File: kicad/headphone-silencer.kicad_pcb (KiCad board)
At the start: 2 copper layers, 61 x 12 mm, 6 parts, among them J1 AudioJack3, J2 AudioJack3

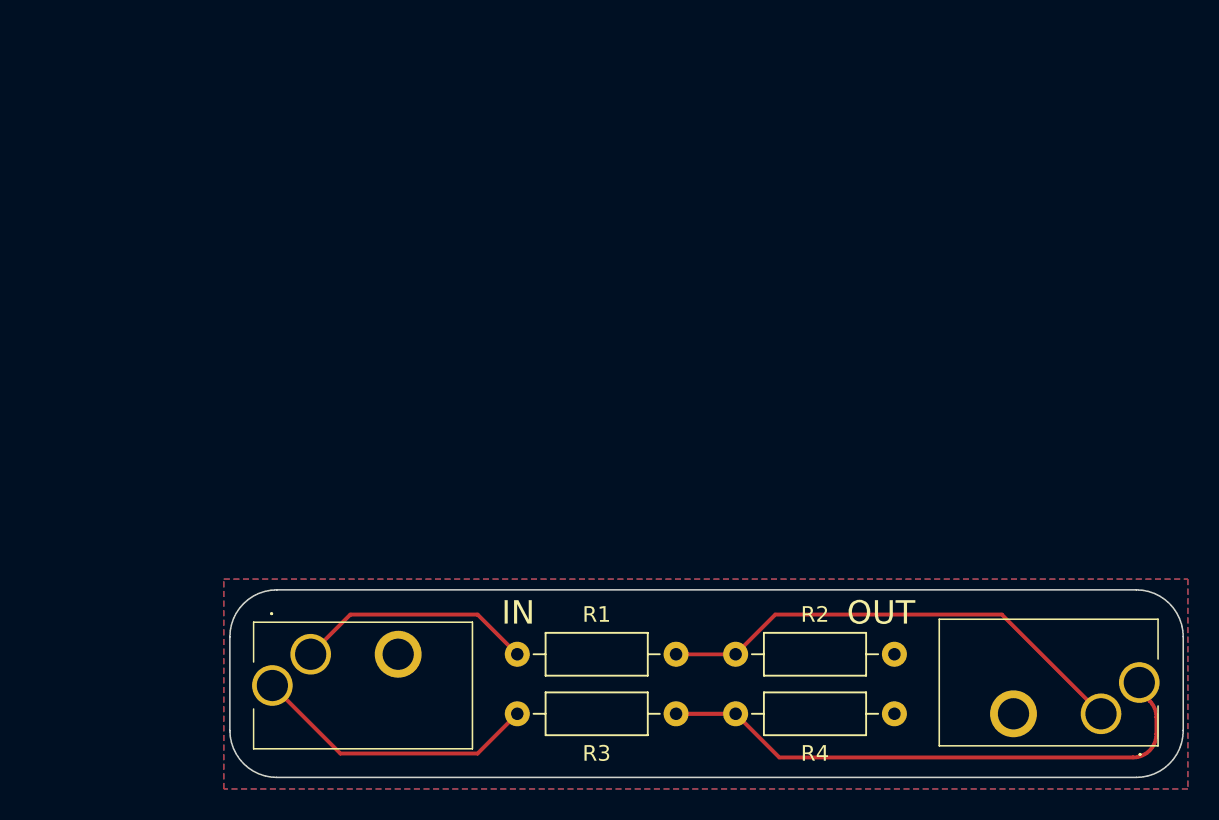
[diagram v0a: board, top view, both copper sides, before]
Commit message: Add pdfs
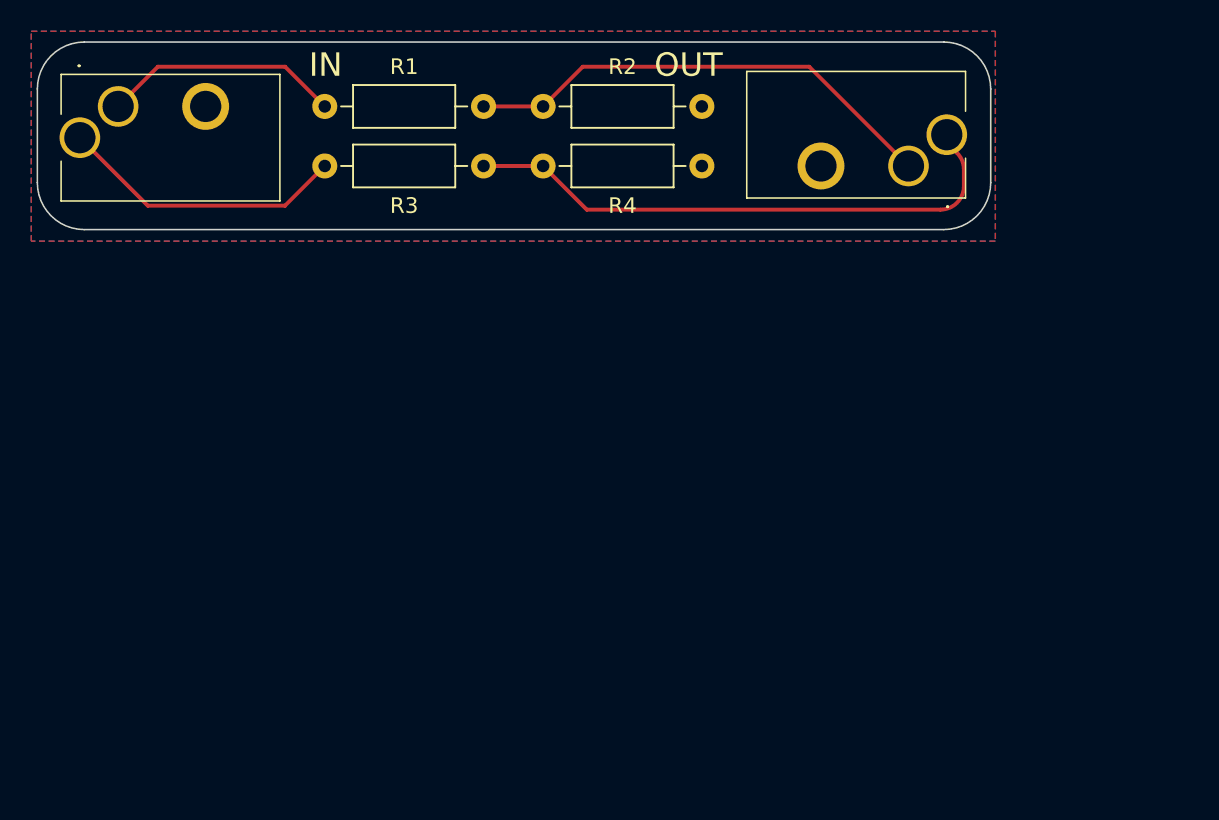
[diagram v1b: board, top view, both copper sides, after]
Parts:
- moved J1 37.2 mm to (44.4, 38.1)
- moved J2 37.2 mm to (99.9, 37.9)
- moved R1 37.2 mm to (60.1, 36.1)
- moved R2 37.2 mm to (74.0, 36.1)
- moved R3 37.2 mm to (60.1, 39.9)
- moved R4 37.2 mm to (74.0, 39.9)
